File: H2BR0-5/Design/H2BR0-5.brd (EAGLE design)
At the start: 60 x 34.6 mm, 62 parts, among them J1 CUI_DEVICES_SJ-3524-SMT-TRCUI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, P2 HEXABIT_X2_P1_P5, U1 STM32G0B1CEU6QFN_B1CEU6_STM-L, U2 AD8232ACPZ-WP, U3 MCP6002, X1 XTALL_CSTCE8M00G52

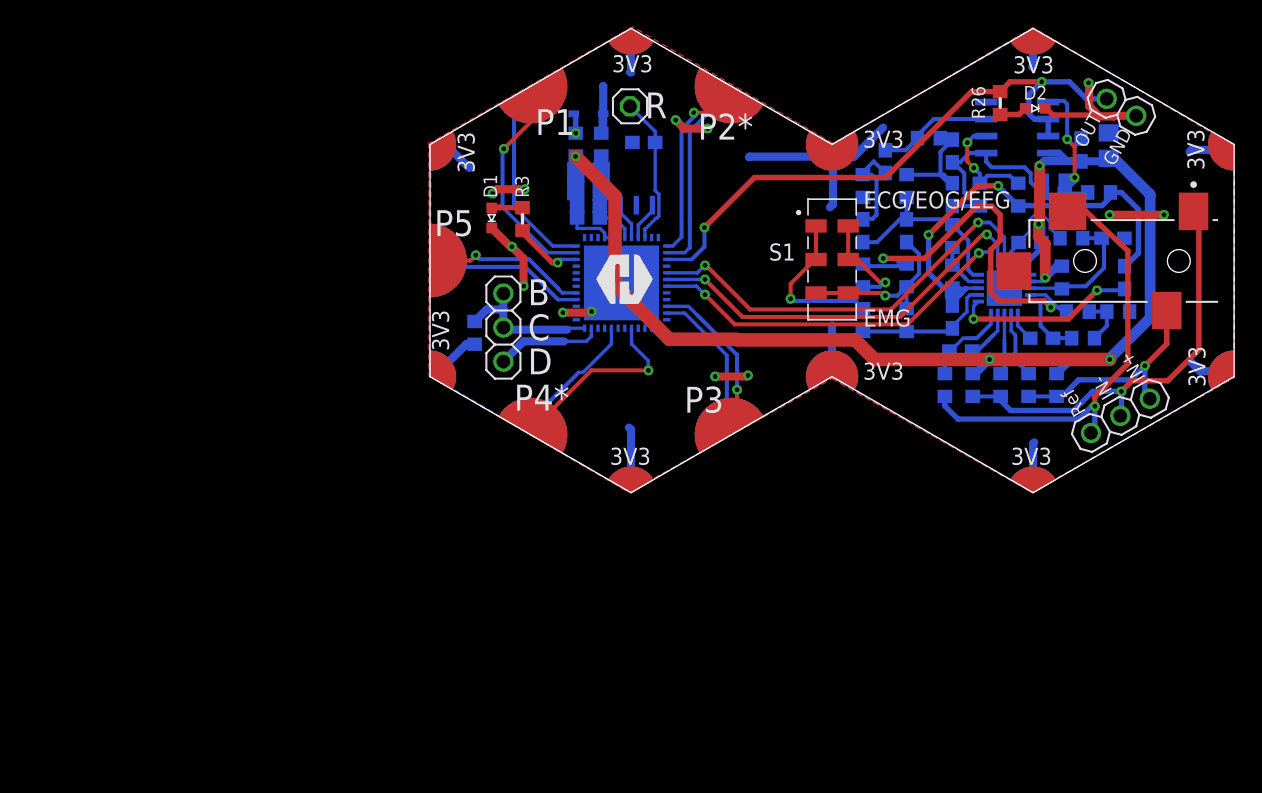
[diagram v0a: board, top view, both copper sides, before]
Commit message: -The final design, all done.
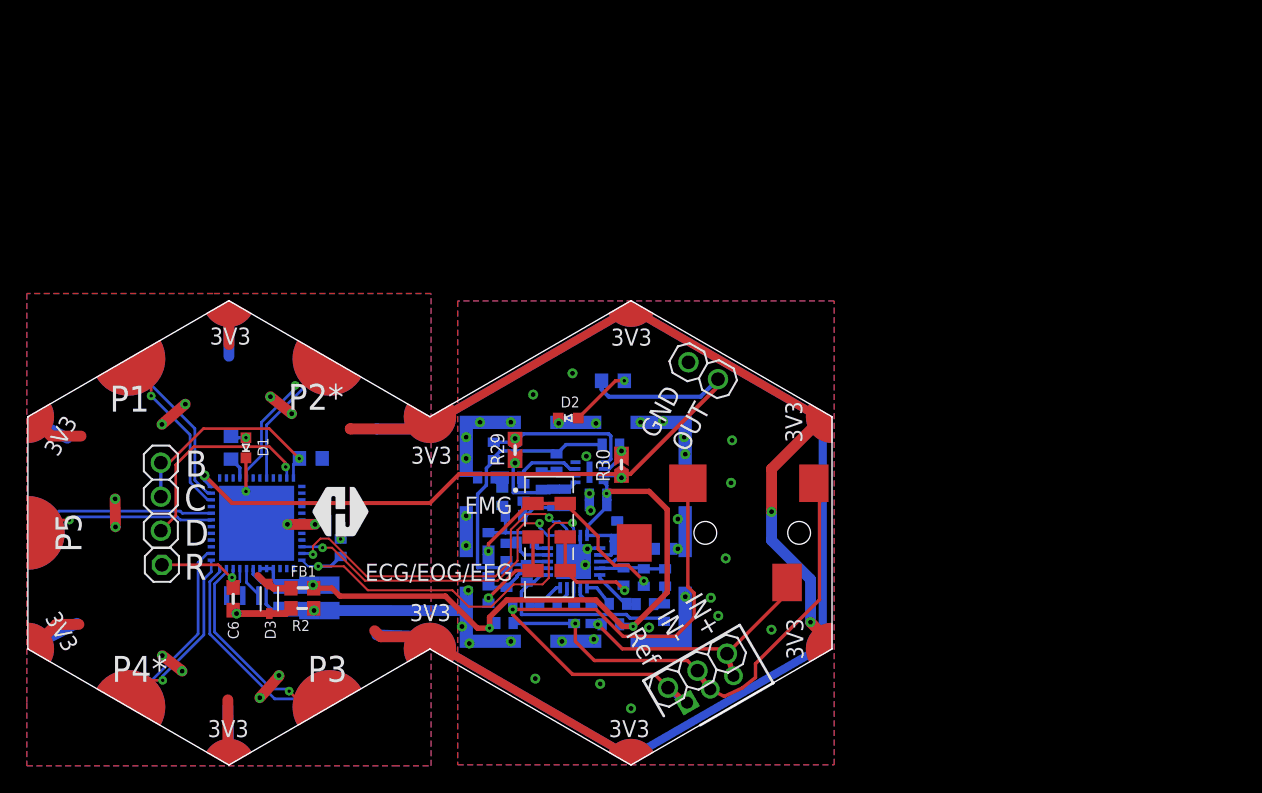
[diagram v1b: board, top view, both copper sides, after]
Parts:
- removed C14: 1uF, HEXABITZ_RCLS:C-0805-POL
- added C5: 1uF, HEXABITZ_RCLS:C-0402
- added J3: 440054-3, HEXABITZ_CONNECTION_PARTS:SHDR3W50P0X200_1X3_800X470X635
- added R28: 100k, HEXABITZ_RCLS:R-0402
- added R29, R30: (no value), HEXABITZ_RCLS:SB-0603
- added R31: 22K, HEXABITZ_RCLS:R-0402
- added SH1: SMS-202C, HEXABITZ_OTHER_PARTS:SMS202F
- C10, C11, C12, C13, C15, C16, C17, C18, C19, C21, C8, C9: device HEXABITZ_RCLS:C-0603 -> HEXABITZ_RCLS:C-0402
- C20: value 1uF -> 100nF; device HEXABITZ_RCLS:C-0603 -> HEXABITZ_RCLS:C-0402
- J1: value CUI_DEVICES_SJ-3524-SMT-TRCUI_DEVICES_SJ-3524-SMT-TR_0_0 -> SJ-3524-SMT-TRU; device HEXABITZ_ICs:CUI_DEVICES_SJ-3524-SMT-TR_0 -> HEXABITZ_ICs:CUI_SJ-3524-SMT
- R10, R11, R12, R13, R14, R15, R16, R17, R18, R19, R20, R21, R22, R23, R24, R25, R4, R5, R6, R7, R8, R9: device HEXABITZ_RCLS:R-0603 -> HEXABITZ_RCLS:R-0402
- R27: value 0R -> 200k; device HEXABITZ_RCLS:R-0603 -> HEXABITZ_RCLS:R-0402
- U2: value AD8232ACPZ-WP -> AD8232ACPZ-R7
- U3: value MCP6002 -> TSV772IQ2T_SEPARATED_SYMBOLSSON50P200X200X60-9N; device HEXABITZ_ICs:SOIC8-N_MC_MCH-L -> HEXABITZ_ICs:SON50P200X200X60-9N
- moved C10 49.8 mm to (7.14, -3.02), turned to 90 degrees
- moved R25 49.1 mm to (4.68, 6.11), turned to 90 degrees
- moved JP1 48.9 mm to (-20.1, -2.38)
- moved C6 45.8 mm to (-14.8, -4.92), flipped to the top, turned to 270 degrees
- moved C20 44.5 mm to (6.27, 6.11), turned to 270 degrees
- moved C15 44.3 mm to (12.5, 2.86), turned to 0 degrees
- moved D3 43.3 mm to (-12.1, -4.92), flipped to the top, turned to 90 degrees
- moved D2 41.8 mm to (10.2, 8.57), turned to 270 degrees
- moved C21 41.6 mm to (16.0, -0.56), turned to 90 degrees
- moved X1 41.4 mm to (-14.0, -4.68), turned to 270 degrees
- moved R2 41.2 mm to (-9.60, -5.64), flipped to the top, turned to 180 degrees
- moved U3 41.0 mm to (11.8, 4.52)
- moved R8 40.7 mm to (17.4, -5.95), turned to 270 degrees
- moved R20 40.2 mm to (6.91, 3.02), turned to 90 degrees
- moved R24 39.8 mm to (9.37, 5.24)
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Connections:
- removed net N$28: C18.2, C19.2, R20.1, R21.2
- removed net N$3 (its old number): C21.1, R4.1, R5.2, U2.18
- removed net REFOUT: C10.1, C13.2, R16.2, R24.2, R25.1, U2.8
- removed net SW: C10.2, R8.2, U2.6
- removed net USART6_RX: P2.PAD_PD1, U1.48
- removed net USART6_TX: P2.PAD_PU1, U1.47
- new net N$11: R18.2, S1.6, S1.7
- new net N$12: C12.2, R14.1, R15.1, S1.1, S1.5
- new net N$14: C9.1, R6.2, U2.20
- new net N$22: C18.2, C19.2, C20.2, R23.1, R29.2, U3.1
- new net N$29: C11.2, U2.4
- new net USART4_RX: P2.PAD_PD3, U1.12
- new net USART4_TX: P2.PAD_PU3, U1.11
- net GND: no longer C14.2, C15.2, C21.2, C8.2, D2.C, JP4.2, R22.1, R5.1, U2.14, U2.16, U2.21, U3.4
- net IN+: now also J3.3
- net IN-: now also J3.2
- net LOD+: now also U1.47; no longer U1.18
- net LOD-: now also U1.46; no longer U1.19
- net N$10: now also R19.1, S1.2, S1.3; no longer R6.2, R7.2, R8.1
- net N$13: now also R15.2, R18.1, R7.1, U2.19; no longer C11.1, U2.4
- net N$16: now also R6.1, R7.2, R8.1; no longer C12.2, R14.2, R15.1, S1.3, S1.7
- net N$17: now also R23.2, R24.2, U3.2; no longer C11.2, R13.1, U2.5
- net N$18: now also C21.1, R4.1, R5.1, U2.18; no longer C13.1, R14.1, R19.1, U2.7
- net N$19: now also C18.1, C19.1, R20.1, R21.2; no longer R18.1, S1.5, S1.6
- net N$2: now also U1.28; no longer U1.46
- net N$20: now also C11.1, R13.1, U2.5; no longer R19.2, S1.1, S1.2
- net N$23: now also C16.1, C17.2, R22.1; no longer D2.A, R26.1
- net N$24: now also C20.1, R25.2, R29.1, U3.5; no longer C16.1, C17.2, R22.2
- net N$25: now also C10.2, C13.2, R16.2, R24.1, R25.1, R28.2, U2.8; no longer C20.2, R25.2, R27.2, U3.5
- net N$26: now also C10.1, R8.2, U2.6; no longer C18.1, C19.1, C20.1, R23.1, R27.1, U3.1
- net N$27: now also D2.A, R26.2; no longer R23.2, R24.1, U3.2
- net N$7: now also C13.1, R14.2, R19.2, U2.7; no longer C9.1, R6.1, U2.20
- net N$9: now also R27.1, R28.1, R30.2, U3.6; no longer R15.2, R18.2, R7.1, U2.19
- net OUT: now also R26.1, R27.2, R30.1, U1.24; no longer R26.2, U1.15, U3.6
- net REF: now also J3.1
- net SDN: now also R31.2, U1.48; no longer U1.17
- net USART1_RX: now also P2.PAD_PD2; no longer P2.PAD_PD4
- net USART1_TX: now also P2.PAD_PU2; no longer P2.PAD_PU4
- net USART2_RX: now also P2.PAD_PD4; no longer P2.PAD_PD2
- net USART2_TX: now also P2.PAD_PU4; no longer P2.PAD_PU2
- net USART3_RX: now also P2.PAD_PD1; no longer P2.PAD_PD3
- net USART3_TX: now also P2.PAD_PU1; no longer P2.PAD_PU3
- net USART5_RX: now also U1.20; no longer U1.40
- net USART5_TX: now also U1.19; no longer U1.41
- net VDD: now also R31.1
- net VDDA: now also C5.1; no longer C14.1
- net VSSA: now also C15.2, C21.2, C5.2, C8.2, D2.C, JP4.2, R22.2, R5.2, SH1.1, SH1.10, SH1.11, SH1.12, SH1.2, SH1.3, SH1.4, SH1.5, SH1.6, SH1.7, SH1.8, SH1.9, U2.14, U2.16, U2.21, U3.4, U3.9
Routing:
- net VDD: track 1.51 -> 98.6 mm, vias 1 -> 3
- net VDDA: track 107.3 -> 61.4 mm, vias 6 -> 4
- net GND: track 90.8 -> 131.2 mm, vias 13 -> 14
- net REFOUT: track 37.2 -> 0.00 mm, vias 2 -> 0
- net N$9: track 31.4 -> 2.91 mm, vias 2 -> 1
- net N$12: track 0.00 -> 17.4 mm, vias 0 -> 2
- net USART6_TX: track 16.3 -> 0.00 mm, vias 1 -> 0
- net USART4_RX: track 0.00 -> 15.8 mm
- net SW: track 15.5 -> 0.00 mm, vias 2 -> 0
- net USART4_TX: track 0.00 -> 15.4 mm, vias 0 -> 1
- net VSSA: track 7.74 -> 23.1 mm, vias 0 -> 39
- net USART6_RX: track 14.9 -> 0.00 mm
- net N$25: track 11.3 -> 23.4 mm, vias 2 -> 0
- net OUT: track 45.3 -> 56.4 mm
- net N$16: track 12.9 -> 2.14 mm, vias 1 -> 0
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- added copper zone on layer 1, net VSSA
- added copper zone on layer 16, net VSSA
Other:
- board text added: "*"
- board text added: "H2BR01-5"
- board text removed: "H2BR01"
